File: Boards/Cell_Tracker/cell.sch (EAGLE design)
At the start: 27 parts, among them T1 Si1013, U2 LMR16020

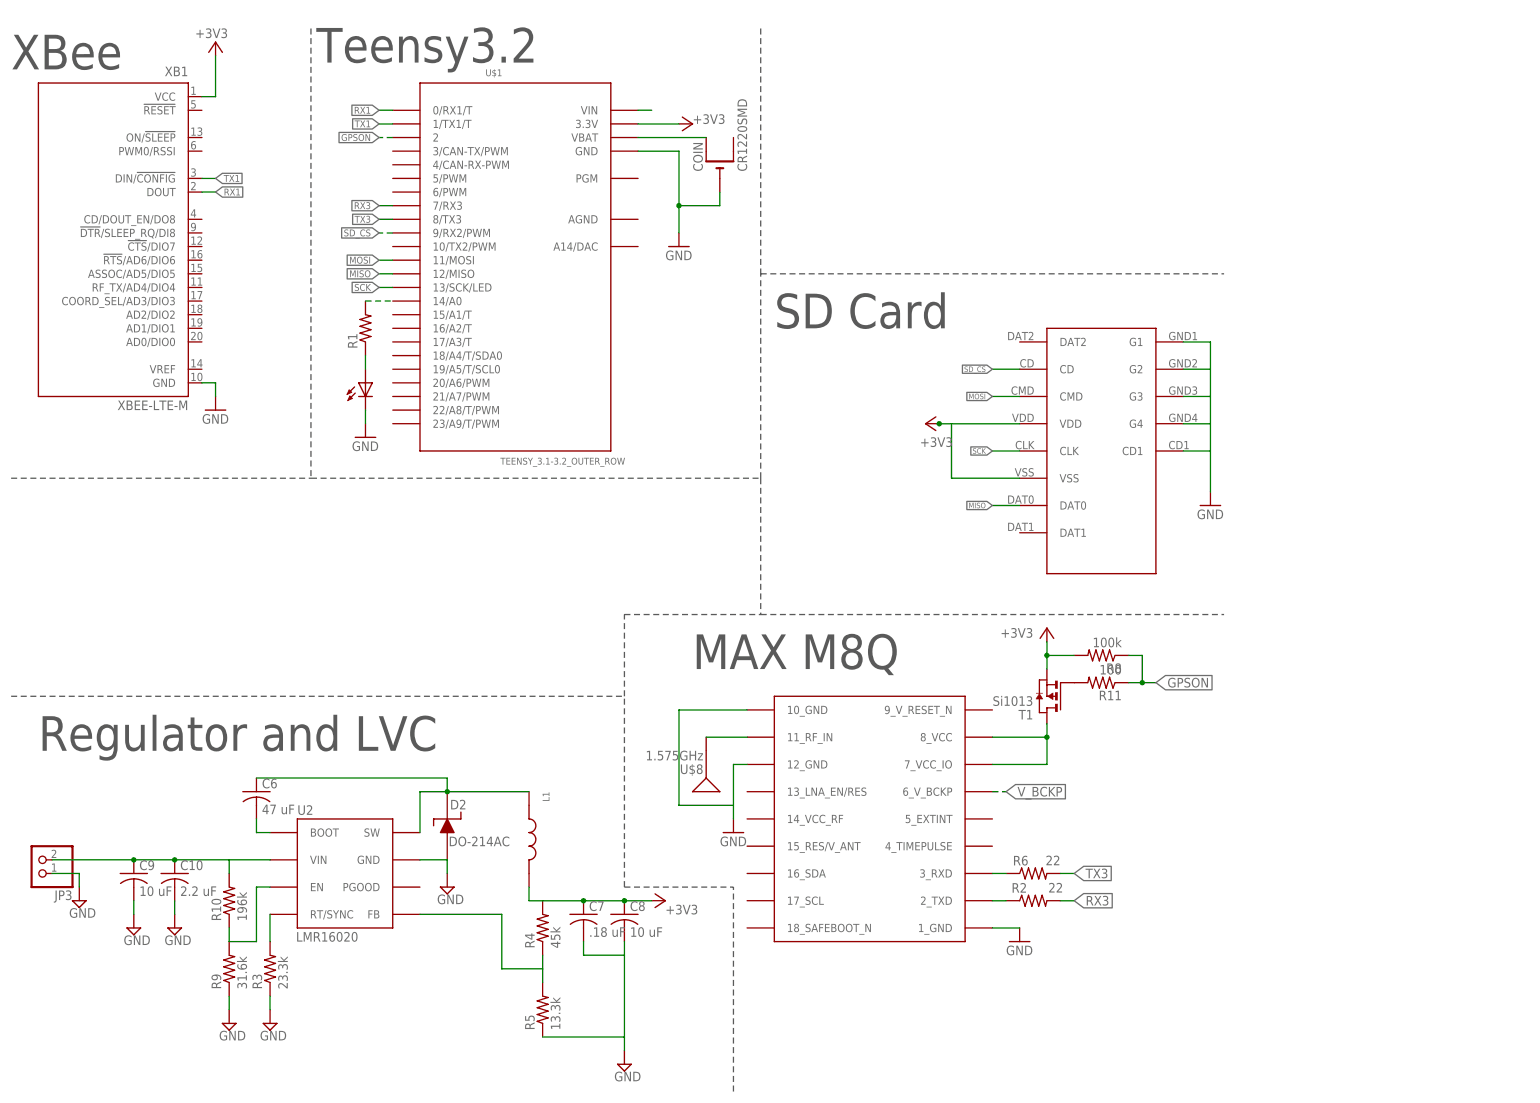
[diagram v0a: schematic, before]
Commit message: cleaned up cell schematic
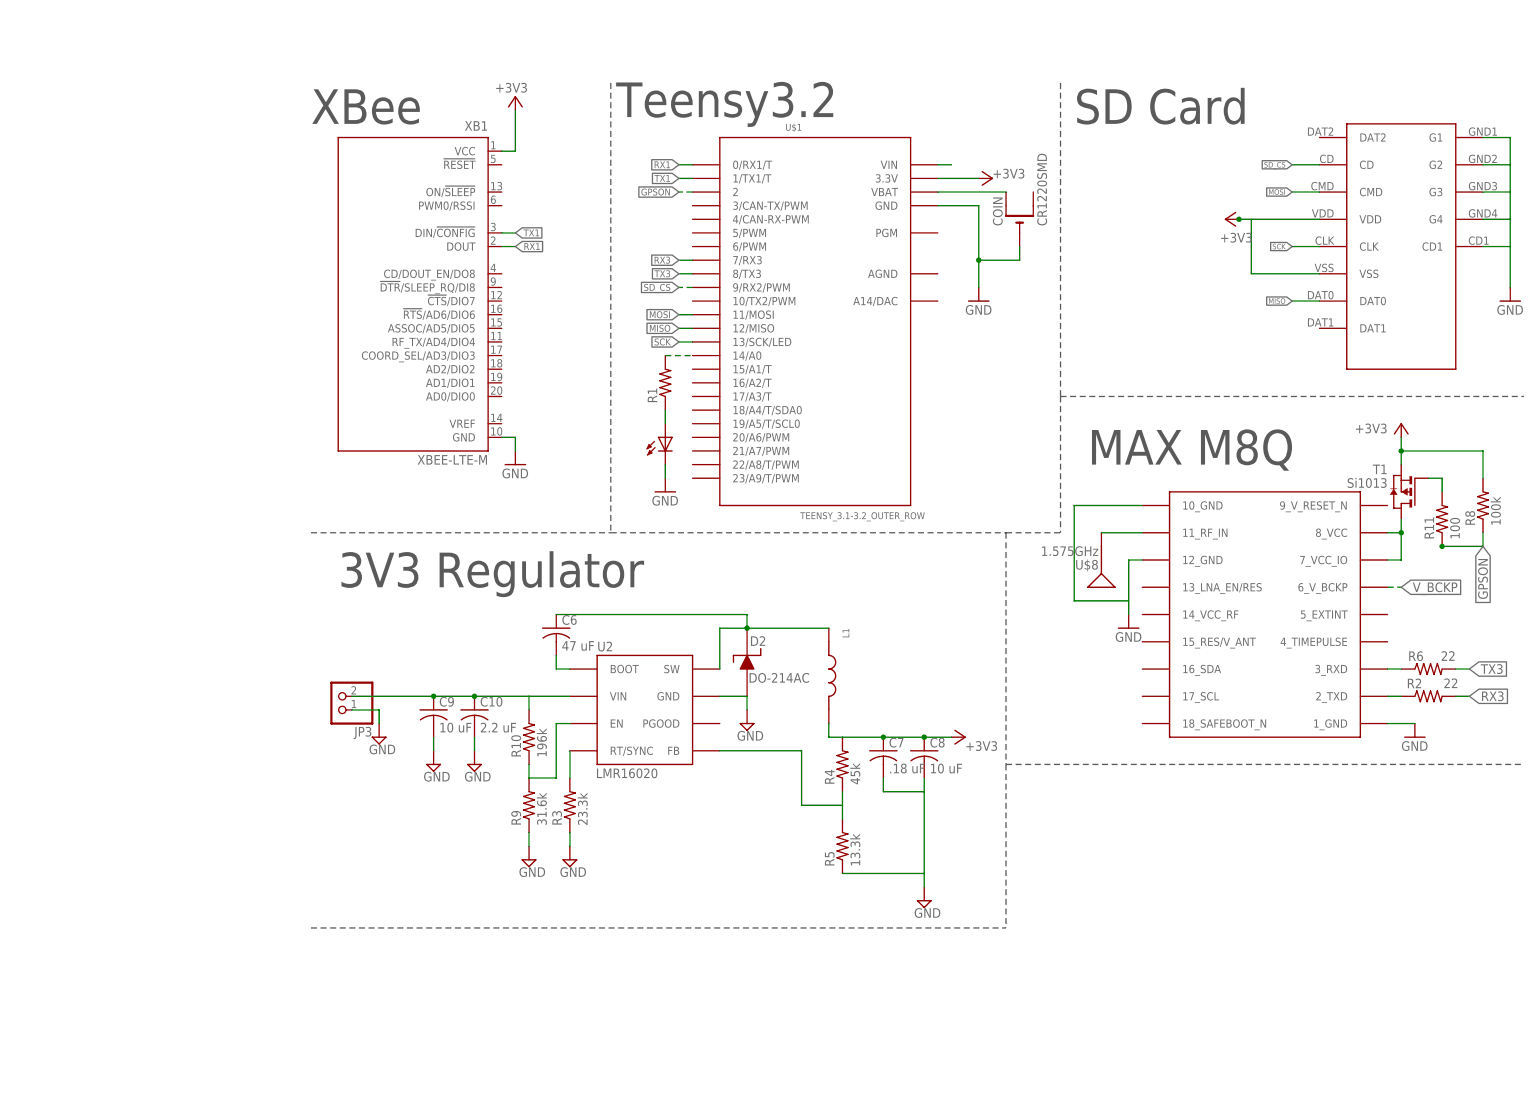
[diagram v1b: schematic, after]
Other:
- note added: "3V3 Regulator"
- note removed: "Regulator and LVC"
- moved on the sheet: C10, C6, C7, C8, C9, COIN, D2, JP3, L1, R1, R10, R11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
